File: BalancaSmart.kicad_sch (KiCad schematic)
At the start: 55 parts, among them J1 Load Cell, J2 Barrel_Jack, Q1 PMOS, Q2 NMOS, Q3 NMOS, Q4 S8050, SW1 SW_Push, U1 HX711-Mod, U2 ADS1115-module, U3 HX-2S-JH20, U4 XL4015

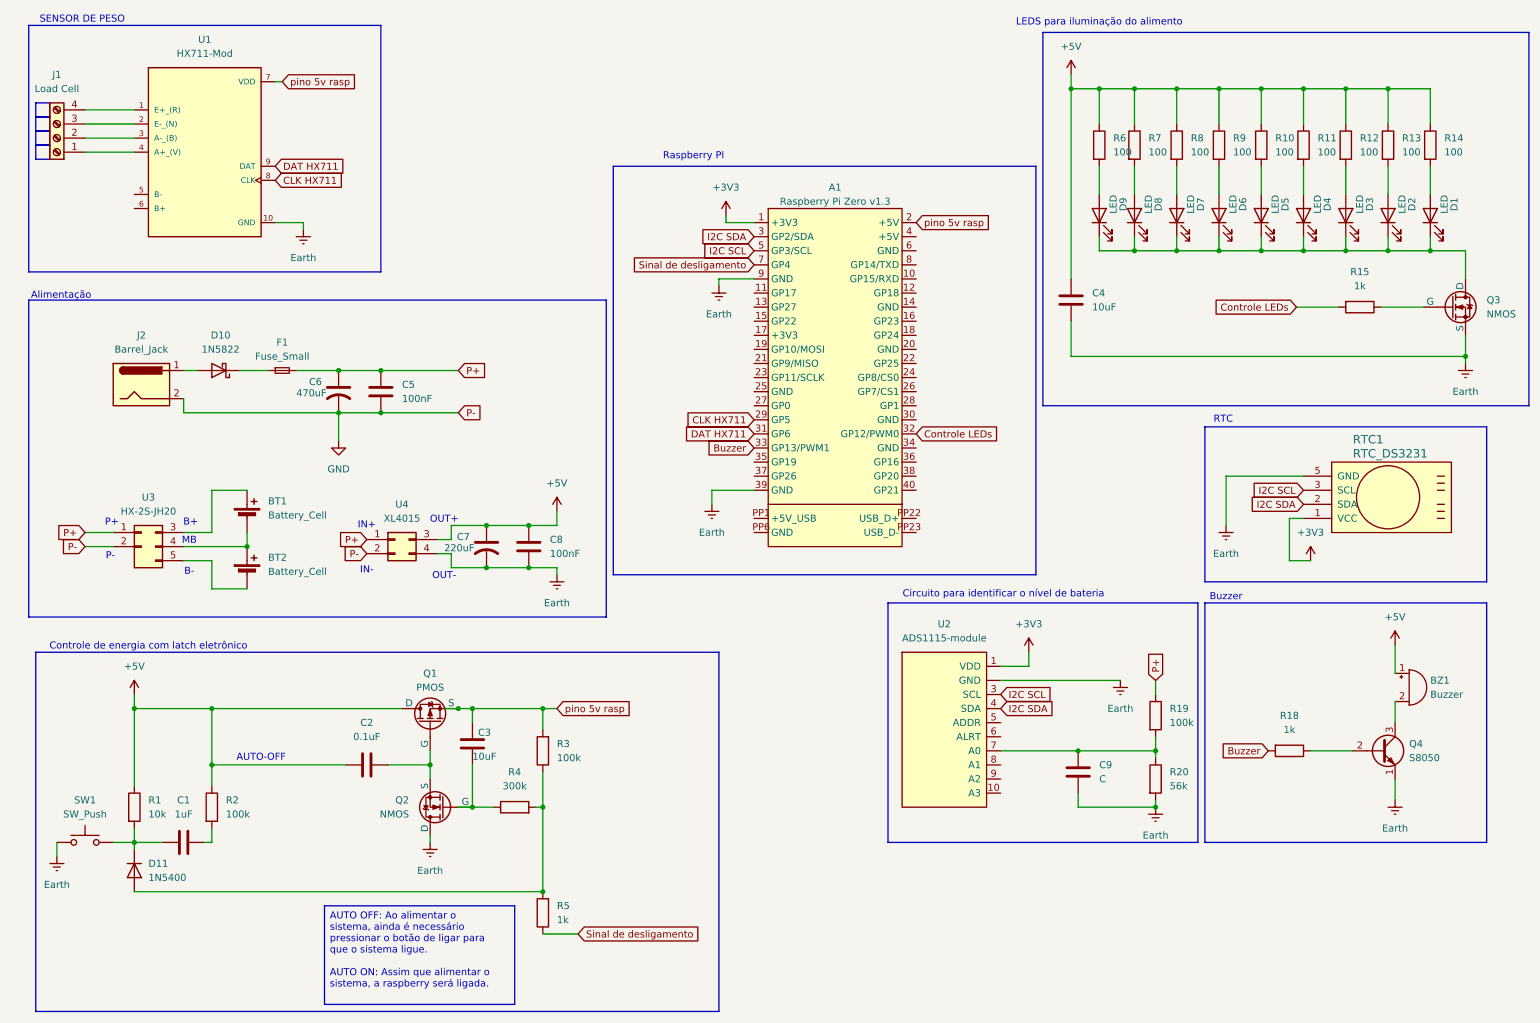
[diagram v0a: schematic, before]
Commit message: layout do circuito dos leds
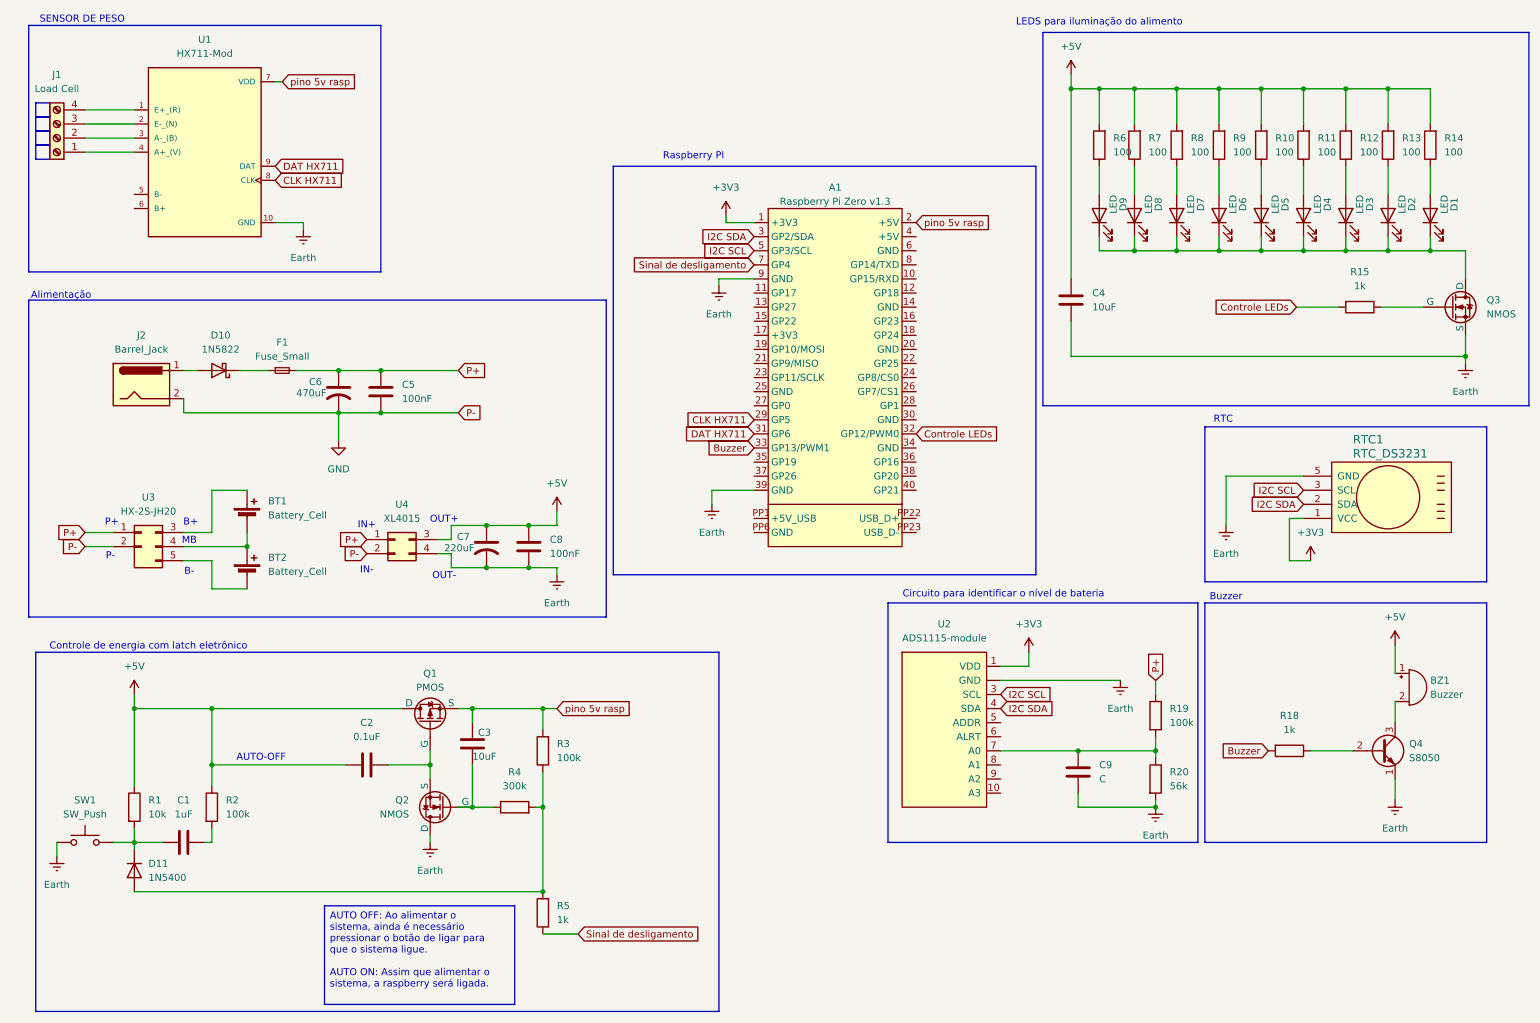
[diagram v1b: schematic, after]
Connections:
- net +5V: now also R10.2, R11.2, R12.2, R13.2, R14.2, R6.2, R7.2, R8.2, R9.2; no longer R10.1, R11.1, R12.1, R13.1, R14.1, R6.1, R7.1, R8.1, R9.1
- net at D5.2 (A): now also R10.1; no longer R10.2
- net at D4.2 (A): now also R11.1; no longer R11.2
- net at D3.2 (A): now also R12.1; no longer R12.2
- net at D2.2 (A): now also R13.1; no longer R13.2
- net at D1.2 (A): now also R14.1; no longer R14.2
- net at D7.2 (A): now also R8.1; no longer R8.2
- net at D6.2 (A): now also R9.1; no longer R9.2
- net at D8.2 (A): now also R7.1; no longer R7.2
- net at D9.2 (A): now also R6.1; no longer R6.2
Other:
- moved on the sheet: R10, R11, R12, R13, R14, R6, R7, R8, R9
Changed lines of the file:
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@@
 	)
 	(junction
-		(at 90.17 139.7)
-		(diameter 0)
-		(color 0 0 0 0)
-	)
-	(junction
 		(at 257.81 57.15)
 		(diameter 0)
@@
 	)
 	(junction
-		(at 92.71 139.7)
-		(diameter 0)
-		(color 0 0 0 0)
-	)
-	(junction
 		(at 234.95 57.15)
 		(diameter 0)
@@
 	)
 	(junction
+		(at 92.71 139.7)
+		(diameter 0)
+		(color 0 0 0 0)
+	)
+	(junction
 		(at 201.93 147.32)
 		(diameter 0)
@@
 	(wire
 		(pts
-			(xy 87.63 139.7) (xy 90.17 139.7)
-		)
-		(stroke
-			(width 0)
-			(type default)
-		)
-	)
-	(wire
-		(pts
 			(xy 107.95 114.3) (xy 102.87 114.3)
 		)
@@
 	(wire
 		(pts
-			(xy 90.17 139.7) (xy 92.71 139.7)
-		)
-		(stroke
-			(width 0)
-			(type default)
-		)
-	)
-	(wire
-		(pts
 			(xy 45.72 118.11) (xy 52.07 118.11)
 		)
@@
 	(wire
 		(pts
+			(xy 90.17 139.7) (xy 92.71 139.7)
+		)
+		(stroke
+			(width 0)
+			(type default)
+		)
+	)
+	(wire
+		(pts
 			(xy 31.75 163.83) (xy 36.83 163.83)
 		)
@@
 	(symbol
 		(lib_id "Device:R")
-		(at 242.57 38.1 0)
+		(at 242.57 38.1 180)
 		(unit 1)
 		(body_style 1)
@@
 					(size 1.27 1.27)
 				)
-				(justify left)
+				(justify right)
 			)
 		)
@@
 					(size 1.27 1.27)
 				)
-				(justify left)
+				(justify right)
 			)
 		)
 		(property "Footprint" "Resistor_THT:R_Axial_DIN0204_L3.6mm_D1.6mm_P7.62mm_Horizontal"
-			(at 240.792 38.1 90)
+			(at 244.348 38.1 90)
 			(hide yes)
 			(show_name no)
@@
 	(symbol
 		(lib_id "Device:R")
-		(at 250.19 38.1 0)
+		(at 250.19 38.1 180)
 		(unit 1)
 		(body_style 1)
@@
 					(size 1.27 1.27)
 				)
-				(justify left)
+				(justify right)
 			)
 		)
@@
 					(size 1.27 1.27)
 				)
-				(justify left)
+				(justify right)
 			)
 		)
 		(property "Footprint" "Resistor_THT:R_Axial_DIN0204_L3.6mm_D1.6mm_P7.62mm_Horizontal"
-			(at 248.412 38.1 90)
+			(at 251.968 38.1 90)
 			(hide yes)
 			(show_name no)
@@
 	(symbol
 		(lib_id "Device:R")
-		(at 234.95 38.1 0)
+		(at 234.95 38.1 180)
 		(unit 1)
 		(body_style 1)
@@
 					(size 1.27 1.27)
 				)
-				(justify left)
+				(justify right)
 			)
 		)
@@
 					(size 1.27 1.27)
 				)
-				(justify left)
+				(justify right)
 			)
 		)
 		(property "Footprint" "Resistor_THT:R_Axial_DIN0204_L3.6mm_D1.6mm_P7.62mm_Horizontal"
-			(at 233.172 38.1 90)
+			(at 236.728 38.1 90)
 			(hide yes)
 			(show_name no)
@@
 	(symbol
 		(lib_id "Device:R")
-		(at 219.71 38.1 0)
+		(at 219.71 38.1 180)
 		(unit 1)
 		(body_style 1)
@@
 					(size 1.27 1.27)
 				)
-				(justify left)
+				(justify right)
 			)
 		)
@@
 					(size 1.27 1.27)
 				)
-				(justify left)
+				(justify right)
 			)
 		)
 		(property "Footprint" "Resistor_THT:R_Axial_DIN0204_L3.6mm_D1.6mm_P7.62mm_Horizontal"
-			(at 217.932 38.1 90)
+			(at 221.488 38.1 90)
 			(hide yes)
 			(show_name no)
@@
 	(symbol
 		(lib_id "Device:R")
-		(at 212.09 38.1 0)
+		(at 212.09 38.1 180)
 		(unit 1)
 		(body_style 1)
@@
 					(size 1.27 1.27)
 				)
-				(justify left)
+				(justify right)
 			)
 		)
@@
 					(size 1.27 1.27)
 				)
-				(justify left)
+				(justify right)
 			)
 		)
 		(property "Footprint" "Resistor_THT:R_Axial_DIN0204_L3.6mm_D1.6mm_P7.62mm_Horizontal"
-			(at 210.312 38.1 90)
+			(at 213.868 38.1 90)
 			(hide yes)
 			(show_name no)
@@
 	(symbol
 		(lib_id "Device:R")
-		(at 205.74 38.1 0)
+		(at 205.74 38.1 180)
 		(unit 1)
 		(body_style 1)
@@
 					(size 1.27 1.27)
 				)
-				(justify left)
+				(justify right)
 			)
 		)
@@
 					(size 1.27 1.27)
 				)
-				(justify left)
+				(justify right)
 			)
 		)
 		(property "Footprint" "Resistor_THT:R_Axial_DIN0204_L3.6mm_D1.6mm_P7.62mm_Horizontal"
-			(at 203.962 38.1 90)
+			(at 207.518 38.1 90)
 			(hide yes)
 			(show_name no)
@@
 	(symbol
 		(lib_id "Device:R")
-		(at 265.43 38.1 0)
+		(at 265.43 38.1 180)
 		(unit 1)
 		(body_style 1)
@@
 					(size 1.27 1.27)
 				)
-				(justify left)
+				(justify right)
 			)
 		)
@@
 					(size 1.27 1.27)
 				)
-				(justify left)
+				(justify right)
 			)
 		)
 		(property "Footprint" "Resistor_THT:R_Axial_DIN0204_L3.6mm_D1.6mm_P7.62mm_Horizontal"
-			(at 263.652 38.1 90)
+			(at 267.208 38.1 90)
 			(hide yes)
 			(show_name no)
@@
 	(symbol
 		(lib_id "Device:R")
-		(at 227.33 38.1 0)
+		(at 227.33 38.1 180)
 		(unit 1)
 		(body_style 1)
@@
 					(size 1.27 1.27)
 				)
-				(justify left)
+				(justify right)
 			)
 		)
@@
 					(size 1.27 1.27)
 				)
-				(justify left)
+				(justify right)
 			)
 		)
 		(property "Footprint" "Resistor_THT:R_Axial_DIN0204_L3.6mm_D1.6mm_P7.62mm_Horizontal"
-			(at 225.552 38.1 90)
+			(at 229.108 38.1 90)
 			(hide yes)
 			(show_name no)
@@
 	(symbol
 		(lib_id "Device:R")
-		(at 257.81 38.1 0)
+		(at 257.81 38.1 180)
 		(unit 1)
 		(body_style 1)
@@
 					(size 1.27 1.27)
 				)
-				(justify left)
+				(justify right)
 			)
 		)
@@
 					(size 1.27 1.27)
 				)
-				(justify left)
+				(justify right)
 			)
 		)
 		(property "Footprint" "Resistor_THT:R_Axial_DIN0204_L3.6mm_D1.6mm_P7.62mm_Horizontal"
-			(at 256.032 38.1 90)
+			(at 259.588 38.1 90)
 			(hide yes)
 			(show_name no)
